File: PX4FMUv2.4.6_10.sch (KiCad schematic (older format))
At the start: 12 parts, among them U1001 BQ24313, U1002 MIC5332

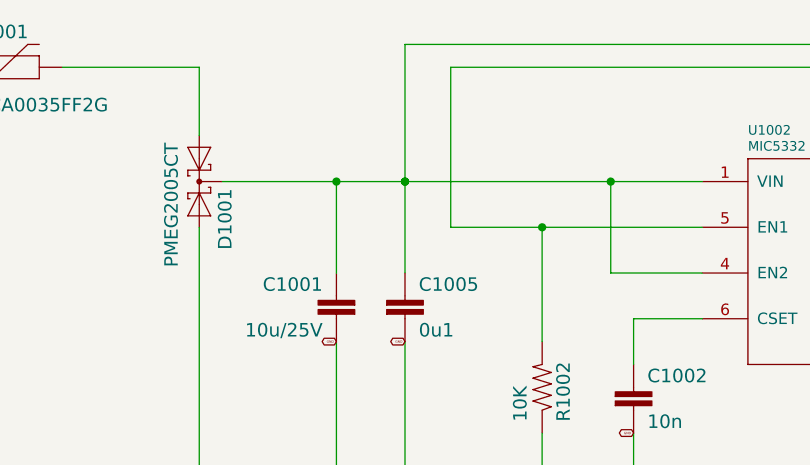
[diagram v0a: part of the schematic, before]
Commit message: removed some things
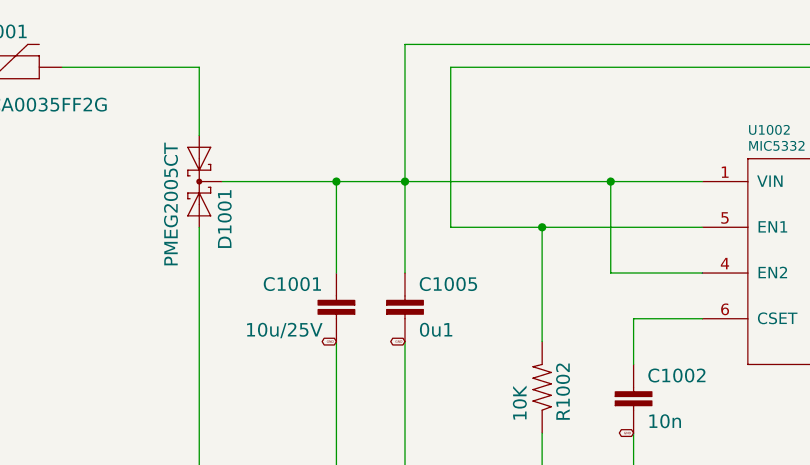
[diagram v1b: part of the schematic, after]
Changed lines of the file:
@@
 EESchema Schematic File Version 4
+LIBS:PX4FMUv2.4.6-cache
 EELAYER 26 0
 EELAYER END
 $Descr User 11797 8268
 encoding utf-8
-Sheet 1 13
+Sheet 11 13
 Title ""
 Date ""
@@
 IO-VDD_5V5
 Connection ~ 4300 2100
-Connection ~ 4600 2100
 Wire Wire Line
 	5600 2900 5600 2700
